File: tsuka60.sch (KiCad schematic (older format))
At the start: 165 parts, among them SW1 SW_Push, U1 ATmega32U4-AU, Y1 Resonator_Small

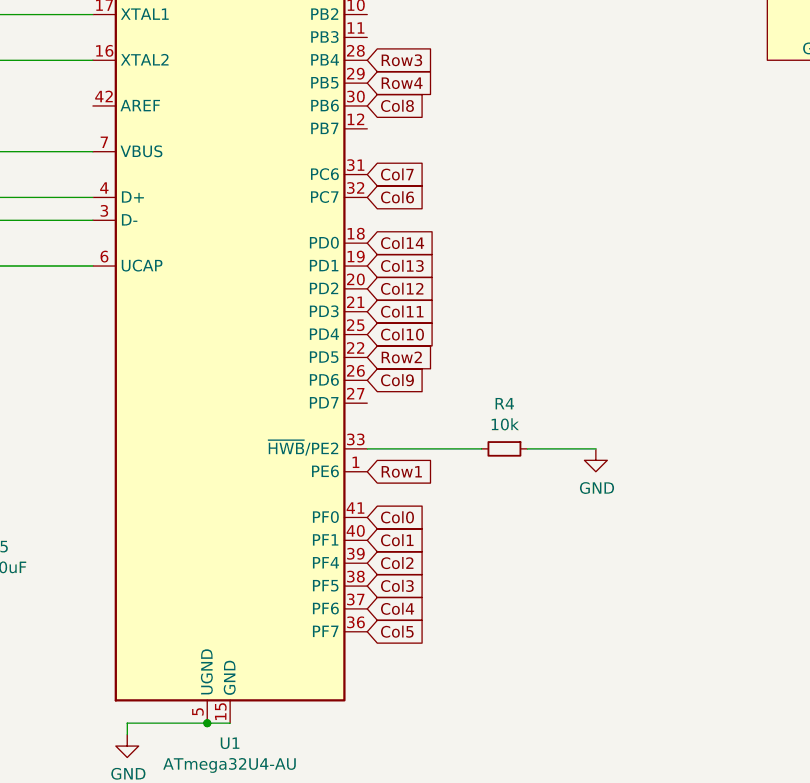
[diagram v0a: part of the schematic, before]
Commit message: more tracing
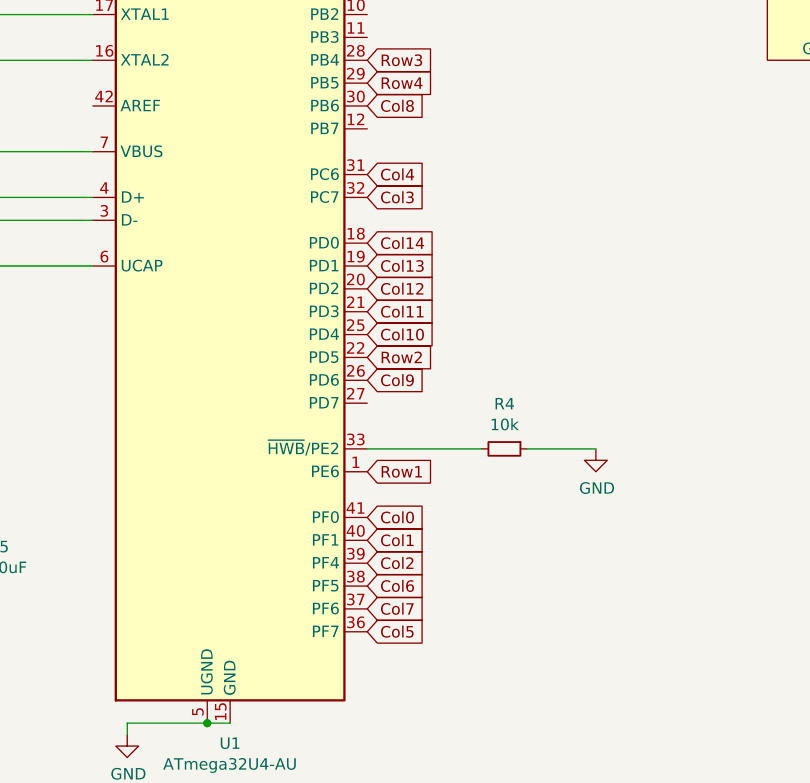
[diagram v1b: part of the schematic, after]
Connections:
- net Col3: now also U1.32 (PC7); no longer U1.38 (PF5)
- net Col4: now also U1.31 (PC6); no longer U1.37 (PF6)
- net Col6: now also U1.38 (PF5); no longer U1.32 (PC7)
- net Col7: now also U1.37 (PF6); no longer U1.31 (PC6)
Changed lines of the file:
@@
 Text GLabel 5750 12950 2    50   Input ~ 0
 Col2
-Text GLabel 5750 13050 2    50   Input ~ 0
+Text GLabel 5750 11350 2    50   Input ~ 0
 Col3
-Text GLabel 5750 13150 2    50   Input ~ 0
+Text GLabel 5750 11250 2    50   Input ~ 0
 Col4
 Text GLabel 5750 13250 2    50   Input ~ 0
 Col5
-Text GLabel 5750 11350 2    50   Input ~ 0
+Text GLabel 5750 13050 2    50   Input ~ 0
 Col6
-Text GLabel 5750 11250 2    50   Input ~ 0
+Text GLabel 5750 13150 2    50   Input ~ 0
 Col7
 Text GLabel 5750 10950 2    50   Input ~ 0
